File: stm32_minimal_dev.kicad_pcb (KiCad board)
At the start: 2 copper layers, 53.3 x 35.6 mm, 33 parts, among them J1 Conn_01x12_Male, J2 Conn_01x12_Male, J3 Conn_01x08_Male, J4 USB_B_Micro, SW1 SW_SPDT, U1 AMS1117-3.3, U2 STM32F103C8T6, Y1 16MHz

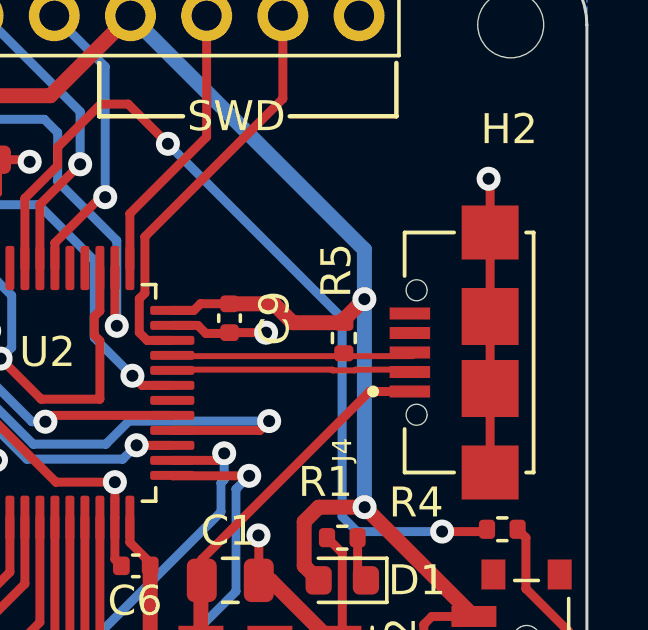
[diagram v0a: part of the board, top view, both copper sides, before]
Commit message: updated files
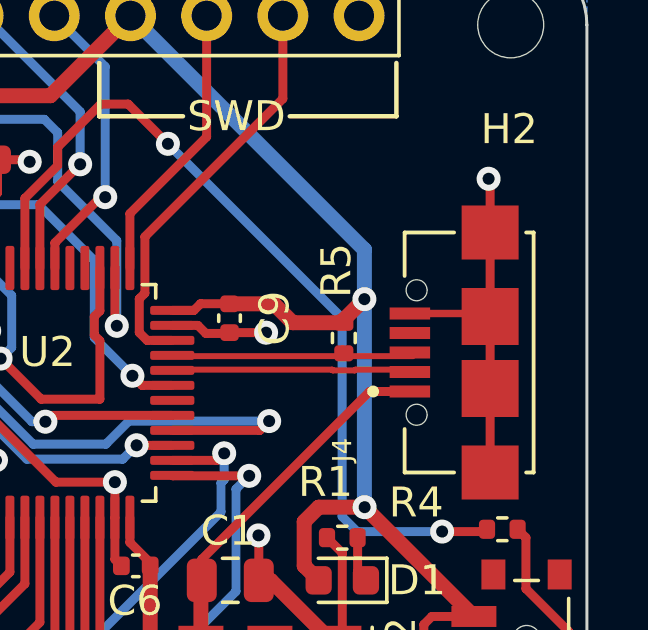
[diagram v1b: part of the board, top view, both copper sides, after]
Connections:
- J4 pad 5: unconnected-(J4-Pad5) -> GND
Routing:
- net GND: track 62.5 -> 65.2 mm
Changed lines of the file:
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@@
       (drillshape 0)
       (scaleselection 1)
-      (outputdirectory "jlcpcb/")
+      (outputdirectory "pcbway/")
     )
   )
@@
   (net 45 "unconnected-(J1-Pad5)")
   (net 46 "unconnected-(J4-Pad4)")
-  (net 47 "unconnected-(J4-Pad5)")
-  (net 48 "/USART1_TX")
-  (net 49 "unconnected-(J1-Pad4)")
-  (net 50 "unconnected-(J1-Pad6)")
-  (net 51 "unconnected-(J1-Pad7)")
-  (net 52 "unconnected-(J3-Pad7)")
-  (net 53 "unconnected-(J1-Pad8)")
+  (net 47 "/USART1_TX")
+  (net 48 "unconnected-(J1-Pad4)")
+  (net 49 "unconnected-(J1-Pad6)")
+  (net 50 "unconnected-(J1-Pad7)")
+  (net 51 "unconnected-(J3-Pad7)")
+  (net 52 "unconnected-(J1-Pad8)")
   (footprint "MountingHole:MountingHole_2.2mm_M2" (layer "F.Cu")
     (at 127.0508 73.66)
@@
       (net 36 "PA8") (pinfunction "Pin_6") (pintype "passive"))
     (pad "7" thru_hole oval (at 0 15.24 180) (size 1.7 1.7) (drill 1) (layers *.Cu *.Mask)
-      (net 52 "unconnected-(J3-Pad7)") (pinfunction "Pin_7") (pintype "passive+no_connect"))
+      (net 51 "unconnected-(J3-Pad7)") (pinfunction "Pin_7") (pintype "passive+no_connect"))
     (pad "8" thru_hole oval (at 0 17.78 180) (size 1.7 1.7) (drill 1) (layers *.Cu *.Mask)
       (net 38 "PA10") (pinfunction "Pin_8") (pintype "passive"))
@@
       (net 18 "PC13") (pinfunction "Pin_3") (pintype "passive"))
     (pad "4" thru_hole oval (at 0 7.62 90) (size 1.7 1.7) (drill 1) (layers *.Cu *.Mask)
-      (net 49 "unconnected-(J1-Pad4)") (pinfunction "Pin_4") (pintype "passive+no_connect"))
+      (net 48 "unconnected-(J1-Pad4)") (pinfunction "Pin_4") (pintype "passive+no_connect"))
     (pad "5" thru_hole oval (at 0 10.16 90) (size 1.7 1.7) (drill 1) (layers *.Cu *.Mask)
       (net 45 "unconnected-(J1-Pad5)") (pinfunction "Pin_5") (pintype "passive+no_connect"))
     (pad "6" thru_hole oval (at 0 12.7 90) (size 1.7 1.7) (drill 1) (layers *.Cu *.Mask)
-      (net 50 "unconnected-(J1-Pad6)") (pinfunction "Pin_6") (pintype "passive+no_connect"))
+      (net 49 "unconnected-(J1-Pad6)") (pinfunction "Pin_6") (pintype "passive+no_connect"))
     (pad "7" thru_hole oval (at 0 15.24 90) (size 1.7 1.7) (drill 1) (layers *.Cu *.Mask)
-      (net 51 "unconnected-(J1-Pad7)") (pinfunction "Pin_7") (pintype "passive+no_connect"))
+      (net 50 "unconnected-(J1-Pad7)") (pinfunction "Pin_7") (pintype "passive+no_connect"))
     (pad "8" thru_hole oval (at 0 17.78 90) (size 1.7 1.7) (drill 1) (layers *.Cu *.Mask)
-      (net 53 "unconnected-(J1-Pad8)") (pinfunction "Pin_8") (pintype "passive+no_connect"))
+      (net 52 "unconnected-(J1-Pad8)") (pinfunction "Pin_8") (pintype "passive+no_connect"))
     (pad "9" thru_hole oval (at 0 20.32 90) (size 1.7 1.7) (drill 1) (layers *.Cu *.Mask)
       (net 40 "PB3") (pinfunction "Pin_9") (pintype "passive"))
@@
       (net 11 "/USART1_RX") (pinfunction "Pin_11") (pintype "passive"))
     (pad "12" thru_hole oval (at 0 27.94 90) (size 1.7 1.7) (drill 1) (layers *.Cu *.Mask)
-      (net 48 "/USART1_TX") (pinfunction "Pin_12") (pintype "passive"))
+      (net 47 "/USART1_TX") (pinfunction "Pin_12") (pintype "passive"))
     (pad "13" thru_hole oval (at 0 30.48 90) (size 1.7 1.7) (drill 1) (layers *.Cu *.Mask)
       (net 3 "+3V3") (pinfunction "Pin_13") (pintype "passive"))
@@
       (net 46 "unconnected-(J4-Pad4)") (pinfunction "4") (pintype "passive+no_connect"))
     (pad "5" smd rect locked (at 1.3 -2.675 90) (size 0.4 1.35) (layers "F.Cu" "F.Paste" "F.Mask")
-      (net 47 "unconnected-(J4-Pad5)") (pinfunction "5") (pintype "passive+no_connect"))
+      (net 2 "GND") (pinfunction "5") (pintype "passive"))
     (pad "S1" smd rect locked (at -4 0 90) (size 1.8 1.9) (layers "F.Cu" "F.Paste" "F.Mask")
       (net 2 "GND") (pinfunction "SHIELD") (pintype "passive"))
@@
       (net 42 "PB5") (pinfunction "PB5") (pintype "bidirectional"))
     (pad "42" smd roundrect (at 0.25 -4.1625) (size 0.3 1.475) (layers "F.Cu" "F.Paste" "F.Mask") (roundrect_rratio 0.25)
-      (net 48 "/USART1_TX") (pinfunction "PB6") (pintype "bidirectional"))
+      (net 47 "/USART1_TX") (pinfunction "PB6") (pintype "bidirectional"))
     (pad "43" smd roundrect (at -0.25 -4.1625) (size 0.3 1.475) (layers "F.Cu" "F.Paste" "F.Mask") (roundrect_rratio 0.25)
       (net 11 "/USART1_RX") (pinfunction "PB7") (pintype "bidirectional"))
@@
   (segment (start 158.2042 78.1558) (end 159.2072 78.1558) (width 0.3) (layer "F.Cu") (net 2))
   (segment (start 166.9136 90.6882) (end 166.9034 90.678) (width 0.3) (layer "F.Cu") (net 2))
+  (segment (start 171.95 83.282) (end 174.525 83.282) (width 0.25) (layer "F.Cu") (net 2))
   (segment (start 165.1508 83.947) (end 165.9102 83.947) (width 0.3) (layer "F.Cu") (net 2))
   (segment (start 169.5844 94.4512) (end 169.5844 94.6908) (width 0.5) (layer "F.Cu") (net 2))
@@
   (segment (start 157.8584 79.8068) (end 157.8584 80.686359) (width 0.3) (layer "F.Cu") (net 2))
   (segment (start 157.8584 80.686359) (end 157.6176 80.927159) (width 0.3) (layer "F.Cu") (net 2))
+  (segment (start 174.525 83.282) (end 174.625 83.382) (width 0.25) (layer "F.Cu") (net 2))
   (segment (start 162.1176 91.4776) (end 162.334 91.694) (width 0.3) (layer "F.Cu") (net 2))
   (segment (start 174.625 80.582) (end 174.625 78.8416) (width 0.3) (layer "F.Cu") (net 2))
@@
   (segment (start 153.3777 78.6892) (end 154.686 78.6892) (width 0.3) (layer "B.Cu") (net 40))
   (segment (start 154.686 78.6892) (end 158.676987 82.680187) (width 0.3) (layer "B.Cu") (net 40))
-  (segment (start 161.640936 79.403823) (end 160.1176 80.927159) (width 0.3) (layer "F.Cu") (net 48))
-  (segment (start 161.794577 79.403823) (end 161.640936 79.403823) (width 0.3) (layer "F.Cu") (net 48))
-  (segment (start 160.1176 80.927159) (end 160.1176 81.7657) (width 0.3) (layer "F.Cu") (net 48))
-  (via (at 161.794577 79.403823) (size 0.8) (drill 0.4) (layers "F.Cu" "B.Cu") (net 48))
-  (segment (start 161.794577 75.053577) (end 161.794577 79.403823) (width 0.3) (layer "B.Cu") (net 48))
-  (segment (start 160.0962 73.3552) (end 161.794577 75.053577) (width 0.3) (layer "B.Cu") (net 48))
+  (segment (start 161.640936 79.403823) (end 160.1176 80.927159) (width 0.3) (layer "F.Cu") (net 47))
+  (segment (start 161.794577 79.403823) (end 161.640936 79.403823) (width 0.3) (layer "F.Cu") (net 47))
+  (segment (start 160.1176 80.927159) (end 160.1176 81.7657) (width 0.3) (layer "F.Cu") (net 47))
+  (via (at 161.794577 79.403823) (size 0.8) (drill 0.4) (layers "F.Cu" "B.Cu") (net 47))
+  (segment (start 161.794577 75.053577) (end 161.794577 79.403823) (width 0.3) (layer "B.Cu") (net 47))
+  (segment (start 160.0962 73.3552) (end 161.794577 75.053577) (width 0.3) (layer "B.Cu") (net 47))
   (zone (net 2) (net_name "GND") (layer "B.Cu") (hatch edge 0.508)
     (connect_pads (clearance 0.508))
